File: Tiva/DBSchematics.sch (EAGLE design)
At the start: 24 parts, among them U1 TPS736XXDRB, Y1 16MHz, Y2 32.768kHz

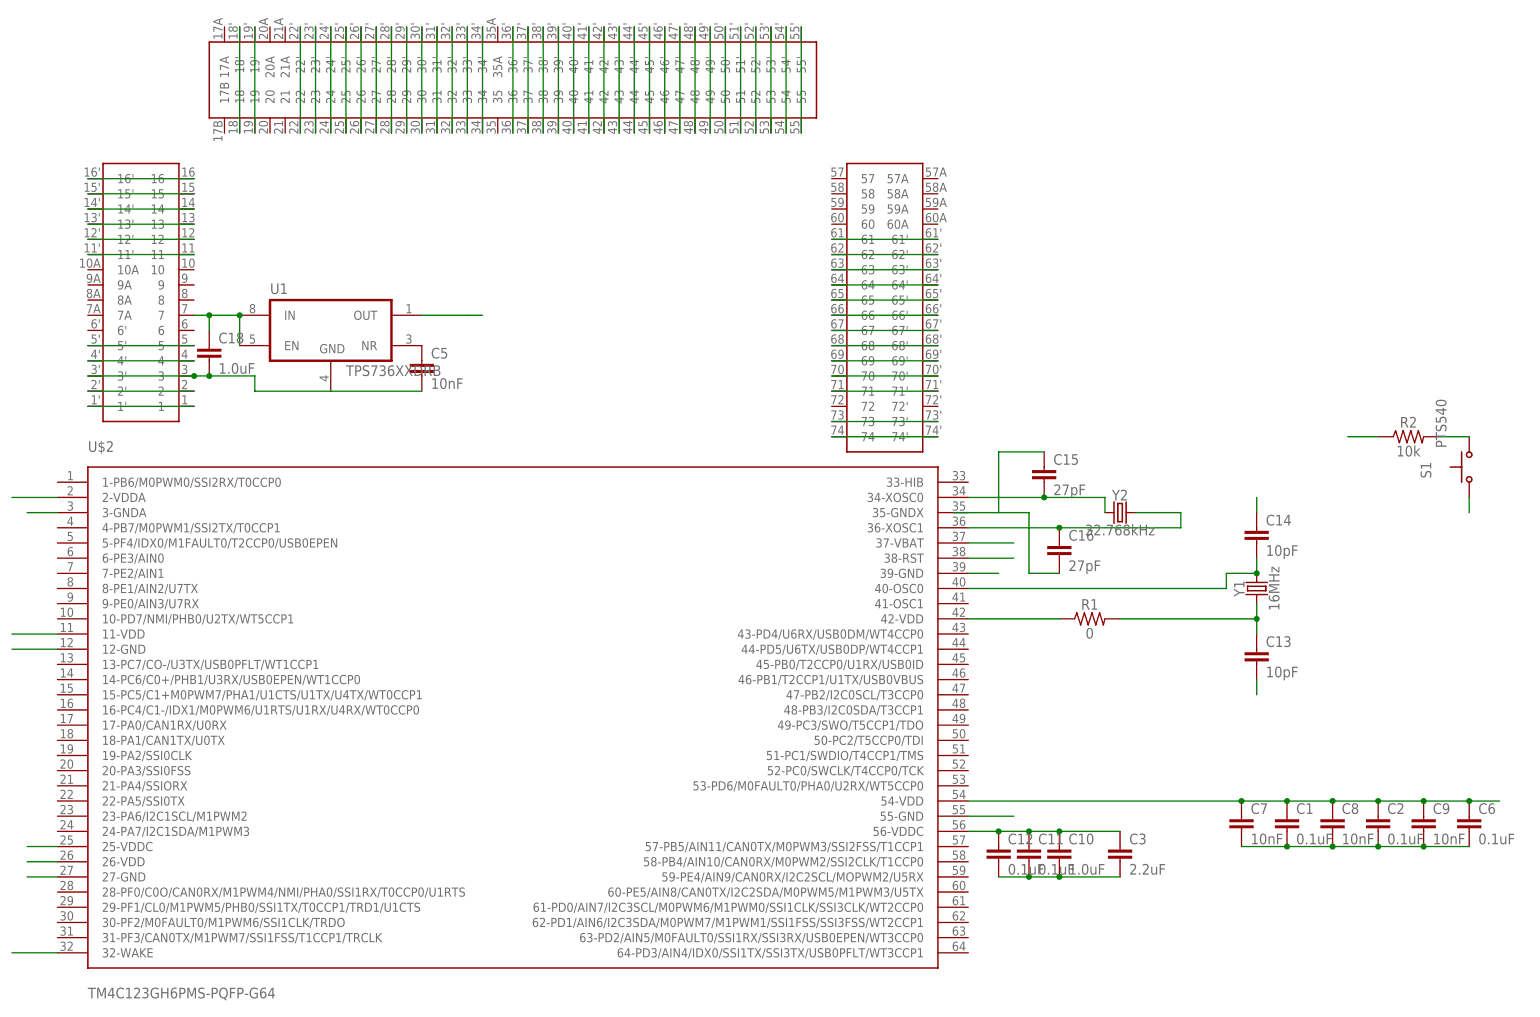
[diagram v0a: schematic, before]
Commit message: Excel Sheet updated
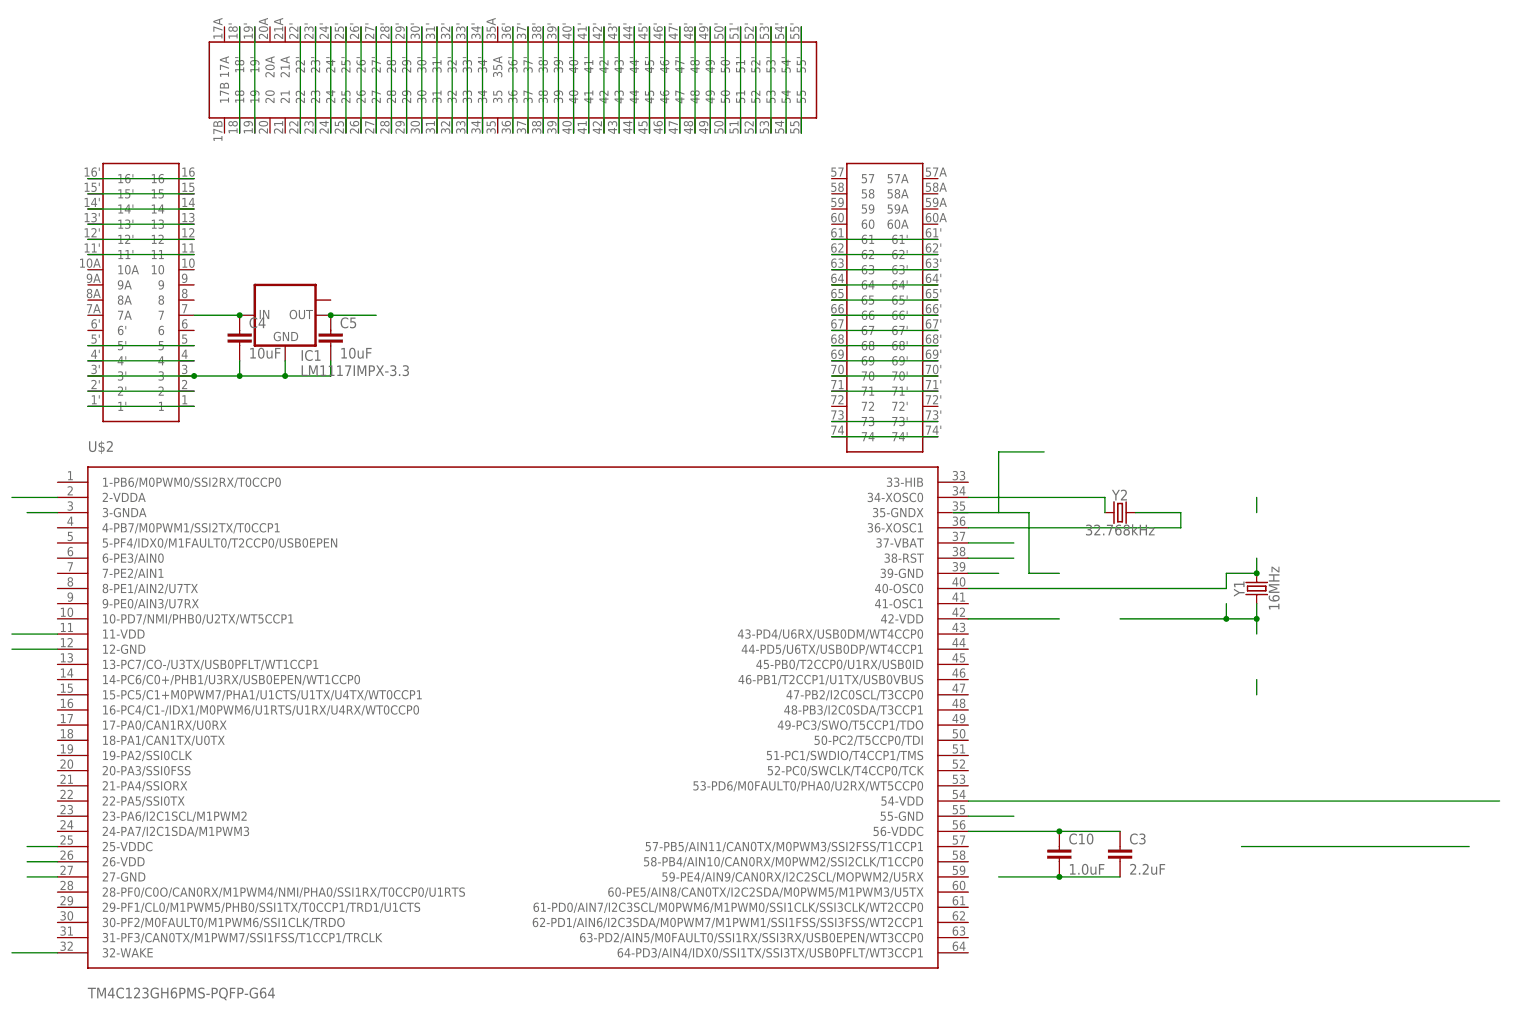
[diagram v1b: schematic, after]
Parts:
- removed C1, C11, C12, C2, C6: 0.1uF, SparkFun-Capacitors:0.1UF-0402-16V-10%
- removed C13, C14: 10pF, SparkFun-Capacitors:10PF-0603-50V-5%
- removed C15, C16: 27pF, SparkFun-Capacitors:27PF-0603-50V-5%
- removed C18: 1.0uF, SparkFun-Capacitors:1.0UF-0402-16V-10%
- removed C7, C8, C9: 10nF, SparkFun-Capacitors:10NF-0603-50V-10%
- removed R1: 0, SparkFun-Resistors:0OHM-0603-1/10W-5%
- removed R2: 10k, SparkFun-Resistors:10KOHM-0603-1/10W-1%
- removed S1: PTS540, switch-ck:PTS540
- removed U1: TPS736XXDRB, texas:TPS736XXDRB
- added C4: 10uF, SparkFun-Capacitors:10UF-1206-6.3V-20%
- added IC1: LM1117IMPX-3.3, lm1117:LM1117IMPX-3.3
- C10: device SparkFun-Capacitors:1.0UF-0402-16V-10% -> SparkFun-Capacitors:1.0UF-1206-50V-10%
- C3: device SparkFun-Capacitors:2.2UF-0603-10V-20% -> SparkFun-Capacitors:2.2UF-1206-50V-10%
- C5: value 10nF -> 10uF; device SparkFun-Capacitors:10NF-0603-50V-10% -> SparkFun-Capacitors:10UF-1206-6.3V-20%
- Y1: device SparkFun-Clocks:CRYSTAL-16MHZSMD-5X3.2 -> SparkFun-Clocks:CRYSTAL-16MHZPTH-HC49US
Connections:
- removed net N$64: C15.1, C16.2
- removed net N$67: C5.1, U1.NR
- net GND: now also C4.2, C5.2, IC1.GND; no longer C1.2, C11.2, C12.2, C13.2, C14.1, C18.2, C2.2, C6.2, C7.2, C8.2, C9.2, S1.P, U1.GND
- net N$25: now also C4.1, IC1.IN; no longer C18.1, U1.EN, U1.IN
- net N$26: no longer C13.1, R1.2
- net N$27: no longer C15.2
- net N$28: no longer C16.1
- net N$3: no longer C14.2
- net RST: no longer R2.1
- net VCC: now also C5.1, IC1.OUT; no longer U1.OUT
- net VDD: no longer C1.1, C2.1, C6.1, C7.1, C8.1, C9.1, R1.1, R2.2, S1.S
- net VDDC: no longer C11.1, C12.1
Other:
- moved on the sheet: C5
